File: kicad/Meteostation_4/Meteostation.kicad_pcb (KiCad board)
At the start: 2 copper layers, 45 x 45 mm, 105 parts, among them J1 TxD, J10 GM+, J11 GM-, J12 SWD, J13 SWC, J2 RxD, J3 BME280_SCL, J4 BME280_SDA, J5 RST, J6 +EXT, J7 -EXT, Q1 5N10, Q2 IRLML6346, Q3 Q_NPN_BEC, T1 HY931147C, U1 STM32F103C8Tx, U2 LMR14206, U3 AD8541, Y2 ECS-250-20-33 25MHz

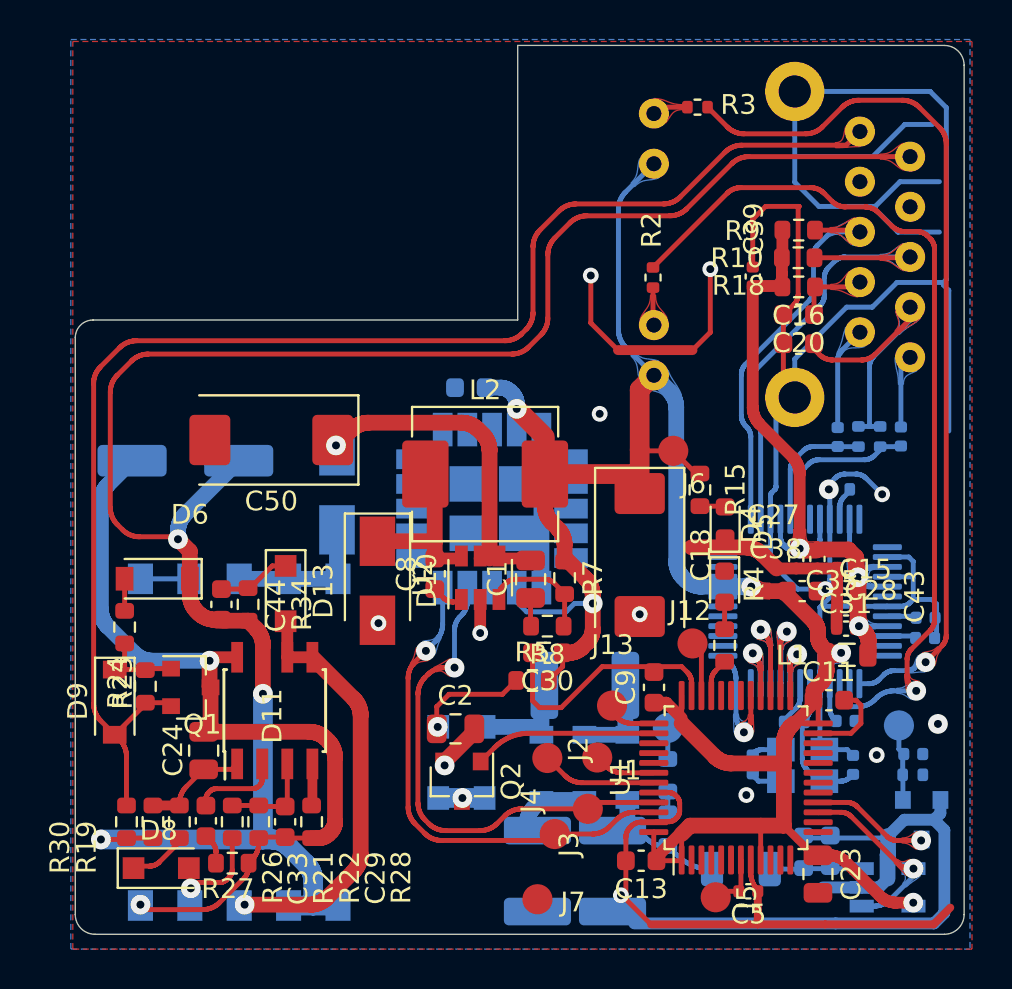
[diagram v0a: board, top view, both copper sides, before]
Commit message: изменено:      kicad/Meteostation_4/Meteostation.kicad_pcb 	изменено:      kicad/Meteostation_4/Meteostation.kicad_pcb-bak 	изменено:      kicad/Meteostation_4/Meteostation.sch 	изменено:      kicad/Meteostation_4/Meteostation.sch-bak
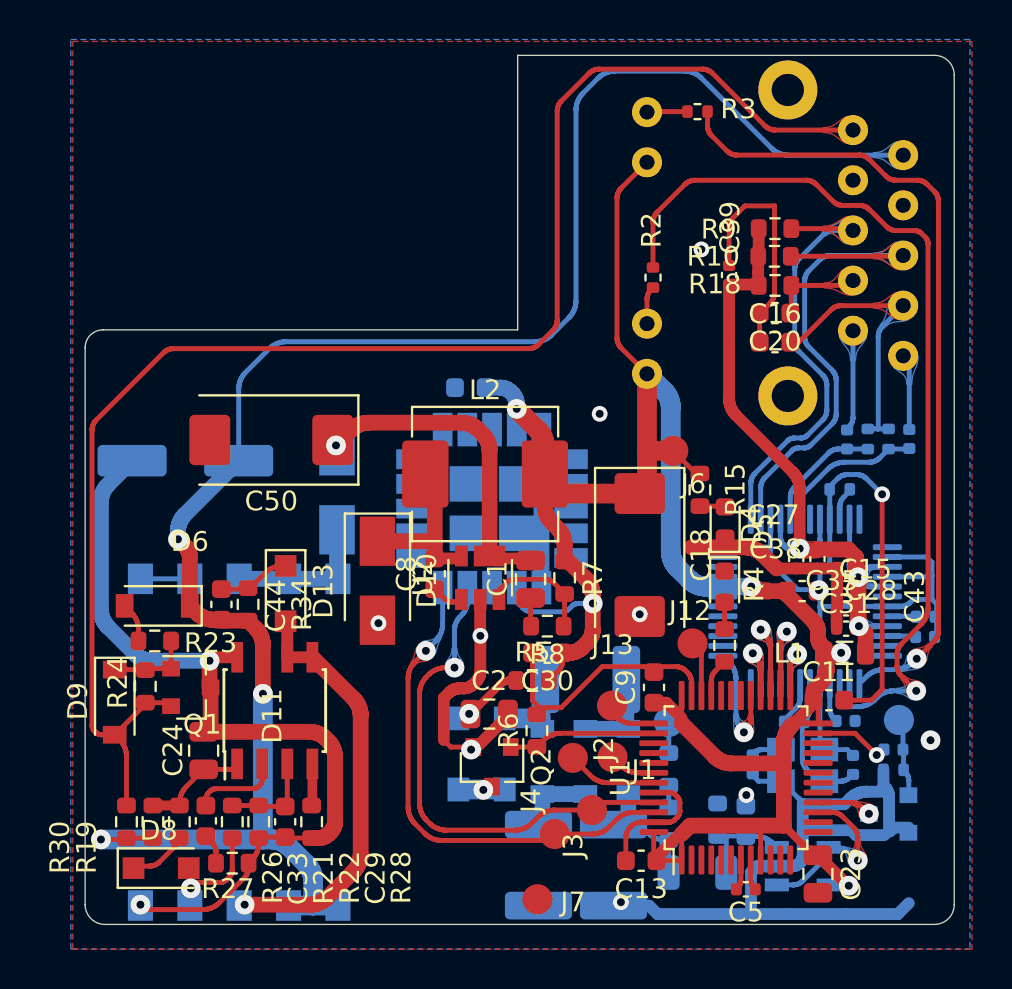
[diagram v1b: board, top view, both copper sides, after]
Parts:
- removed J5: RST, My-library:SMD-CONN
- added R6: 100k, Resistor_SMD:R_0603_1608Metric, F.Cu at (42.5, 94.6)
- moved R16 4.65 mm to (51.6, 99.1)
- moved C22 4.54 mm to (53.0, 99.2)
- moved U3 4.43 mm to (55.9, 101.5)
- moved R13 2.21 mm to (50.6, 101.8)
- moved C2 1.87 mm to (40.1, 93.8)
- moved Q3 1.69 mm to (60.3, 98.8), turned to 180 degrees
- moved Q2 1.69 mm to (40.2, 96.4)
- moved R23 1.68 mm to (23.1, 90.0), turned to 180 degrees
- moved D6 1.38 mm to (23.2, 88.3)
- moved J2 1.29 mm to (44.3, 96.0)
- moved C16 1.20 mm to (54.5, 74.9)
- moved C20 1.20 mm to (54.5, 73.5)
- moved R10 1.20 mm to (54.5, 70.6)
- moved R18 1.20 mm to (54.5, 72.0)
- moved R9 1.20 mm to (54.5, 69.2)
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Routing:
- net GND: track 245.2 -> 167.0 mm, vias 14 -> 12
- net Net-(C19-Pad1): track 99.8 -> 93.8 mm
- net Net-(D9-Pad2): track 72.3 -> 77.7 mm
- net Net-(D3-Pad25): track 44.6 -> 41.0 mm
- net +3.3VDAC: track 120.3 -> 117.5 mm
- net Pulse: track 5.95 -> 3.17 mm
- net Net-(C2-Pad1): track 5.73 -> 3.11 mm
- net Net-(D3-Pad2): track 23.5 -> 25.9 mm
- net Net-(D3-Pad27): track 45.2 -> 47.5 mm
- net Net-(D3-Pad1): track 20.2 -> 22.2 mm
- net PWR: track 9.25 -> 7.47 mm
- net Net-(C5-Pad2): track 2.97 -> 1.56 mm
- net Net-(J2-Pad1): track 5.85 -> 4.57 mm
- net Net-(C17-Pad1): track 6.89 -> 5.92 mm
- net Net-(C20-Pad1): track 3.80 -> 4.65 mm
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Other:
- board size 45 x 45 mm -> 44 x 44 mm
